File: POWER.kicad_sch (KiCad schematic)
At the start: 49 parts, among them J3 Conn_01x02, Q1 2N7002LT3G, Q3 2N7002LT3G, Q7 2N7002LT3G, Q8 2N7002LT3G, U2 TPS62933, U3 TMP300, U6 DRV8428, U8 DRV8220DSGR-8p

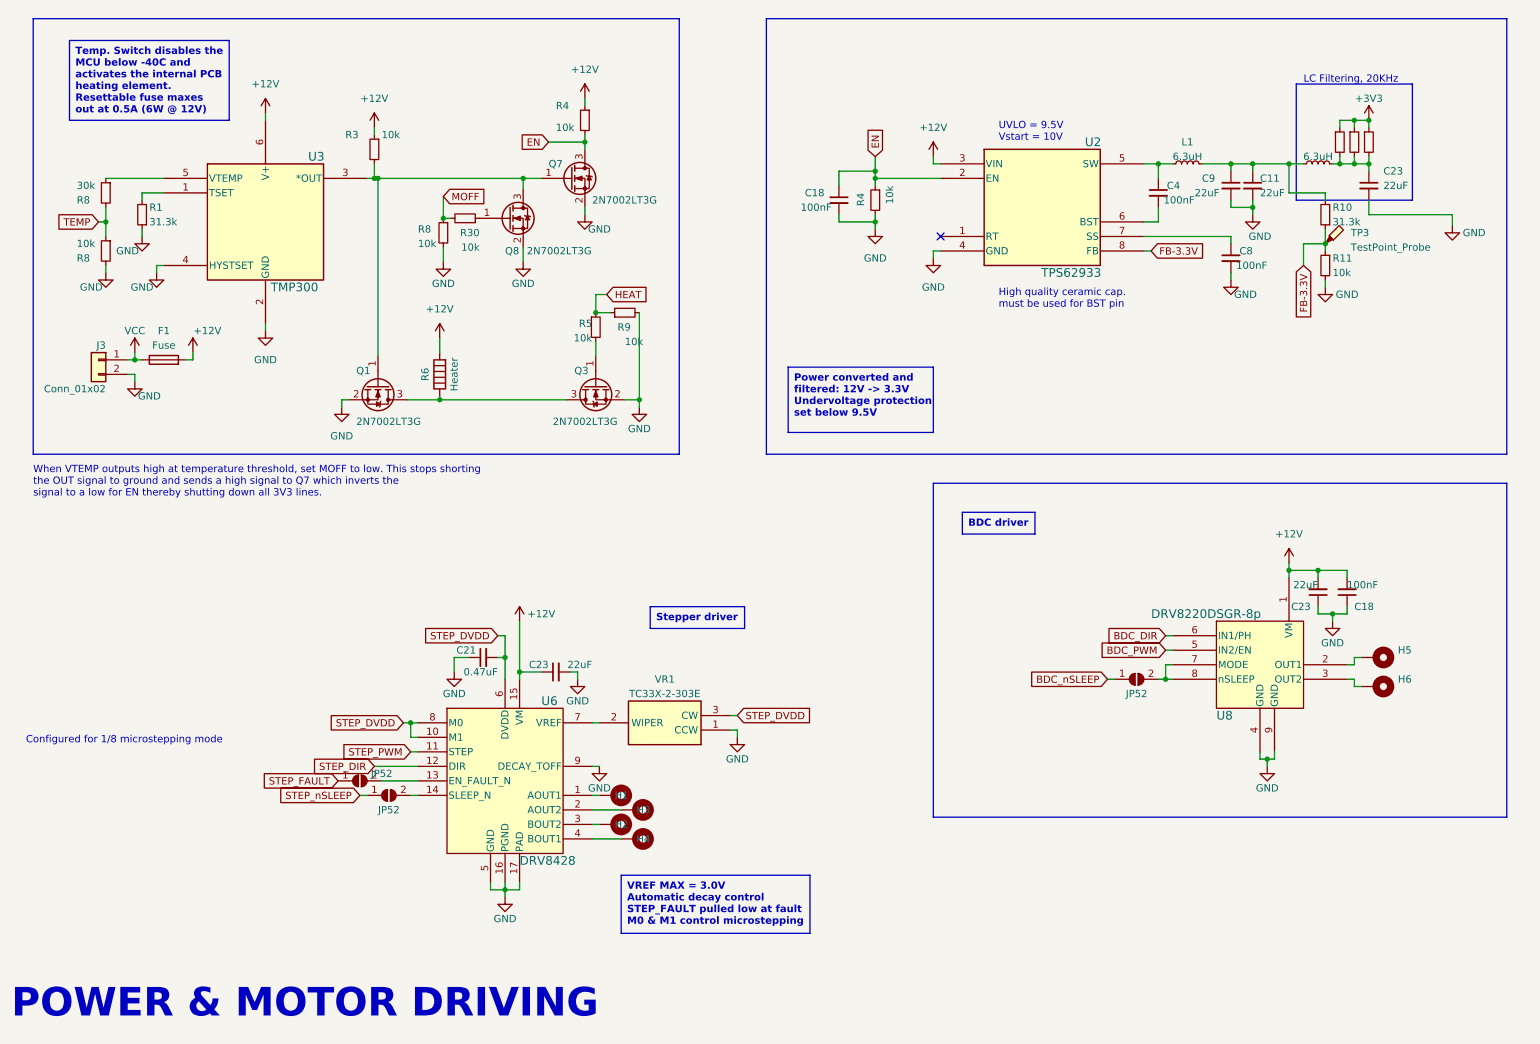
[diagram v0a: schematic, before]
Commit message: Add files via upload
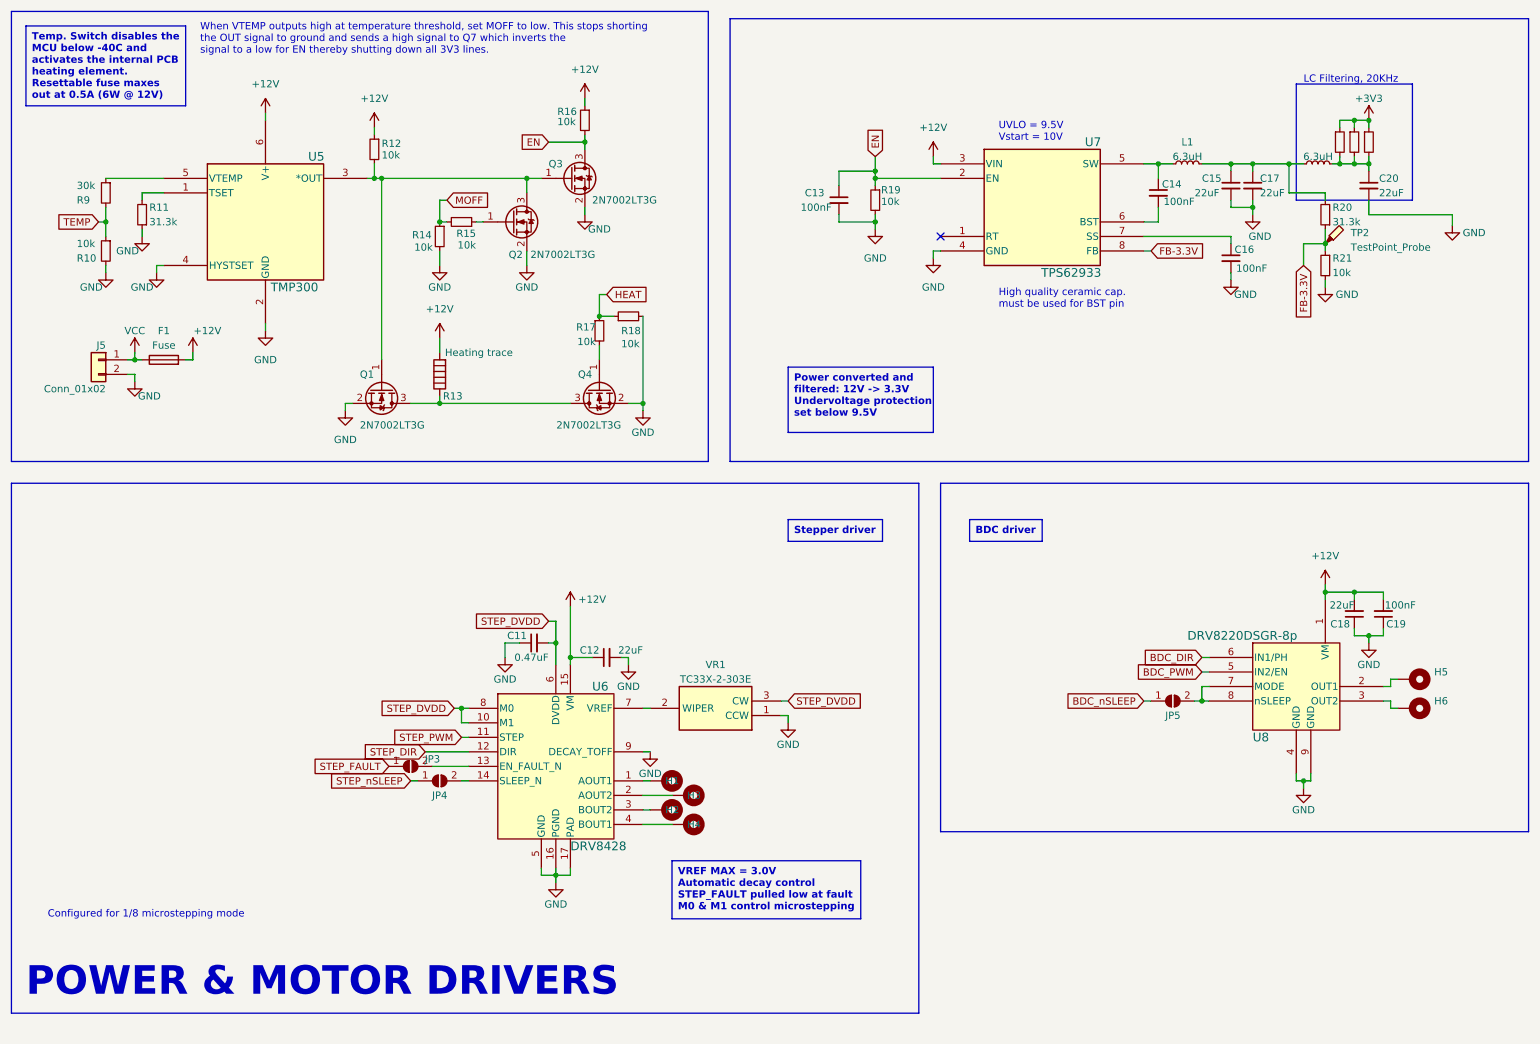
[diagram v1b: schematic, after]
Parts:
- R13: renamed from R6; value Heater -> Heating trace
- renumbered C21 to C11, C23 to C12, C18 to C13, C4 to C14, C9 to C15, C8 to C16, C11 to C17, C23 to C18, C18 to C19, C23 to C20, J3 to J5, JP52 to JP3, JP52 to JP4, JP52 to JP5, Q8 to Q2, Q7 to Q3, Q3 to Q4, R8 to R10, R1 to R11, R3 to R12, R8 to R14, R30 to R15, R4 to R16, R5 to R17, R9 to R18, R4 to R19, R10 to R20, R11 to R21, R7 to R22, R7 to R23, R7 to R24, R8 to R9, TP3 to TP2, U3 to U5, U2 to U7
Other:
- note added: "POWER & MOTOR DRIVERS"
- note removed: "POWER & MOTOR DRIVING"
- moved on the sheet: C11, C12, C18, C19, H1, H2, H3, H4, H5, H6, JP3, JP4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
